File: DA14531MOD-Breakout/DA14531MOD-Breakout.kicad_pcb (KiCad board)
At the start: 2 copper layers, 30.1 x 30 mm, 3 parts, among them J1 Conn_01x07, J2 Conn_01x07, U1 DA14531MOD-00F01002

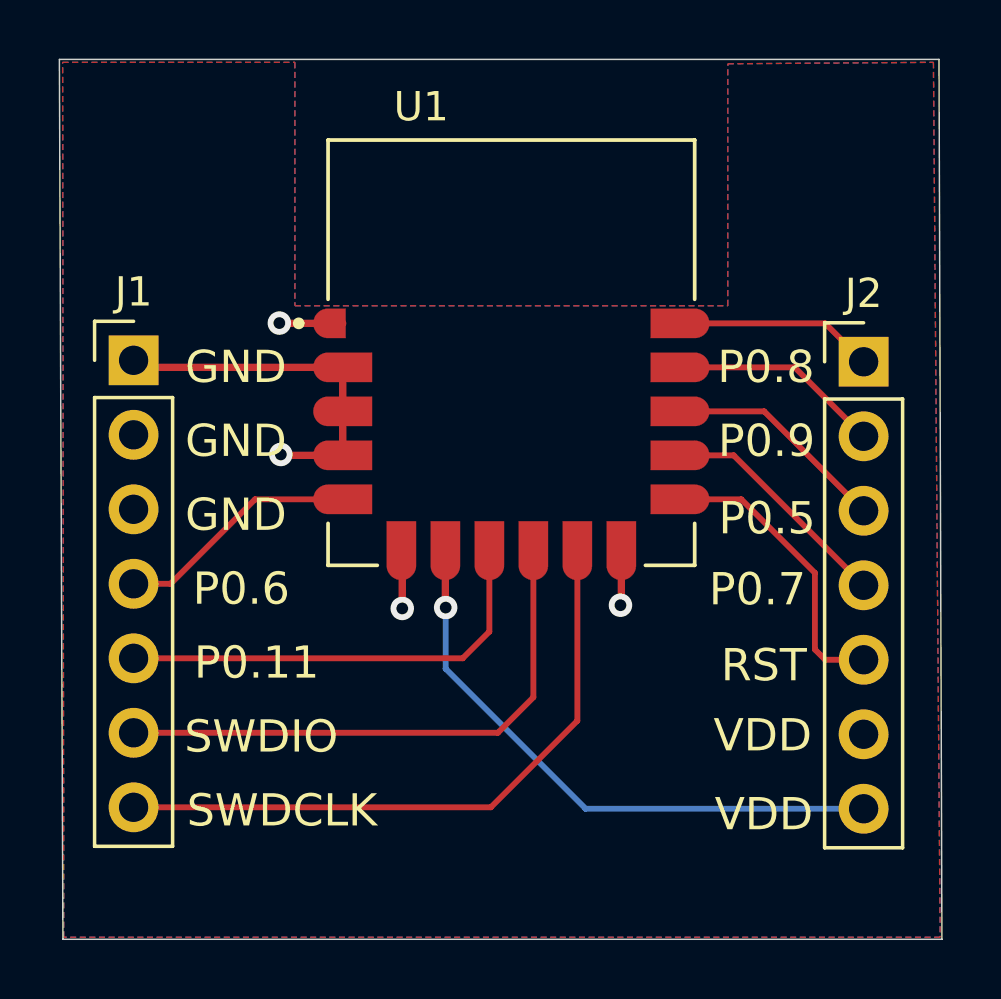
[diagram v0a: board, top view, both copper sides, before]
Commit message: finetuning
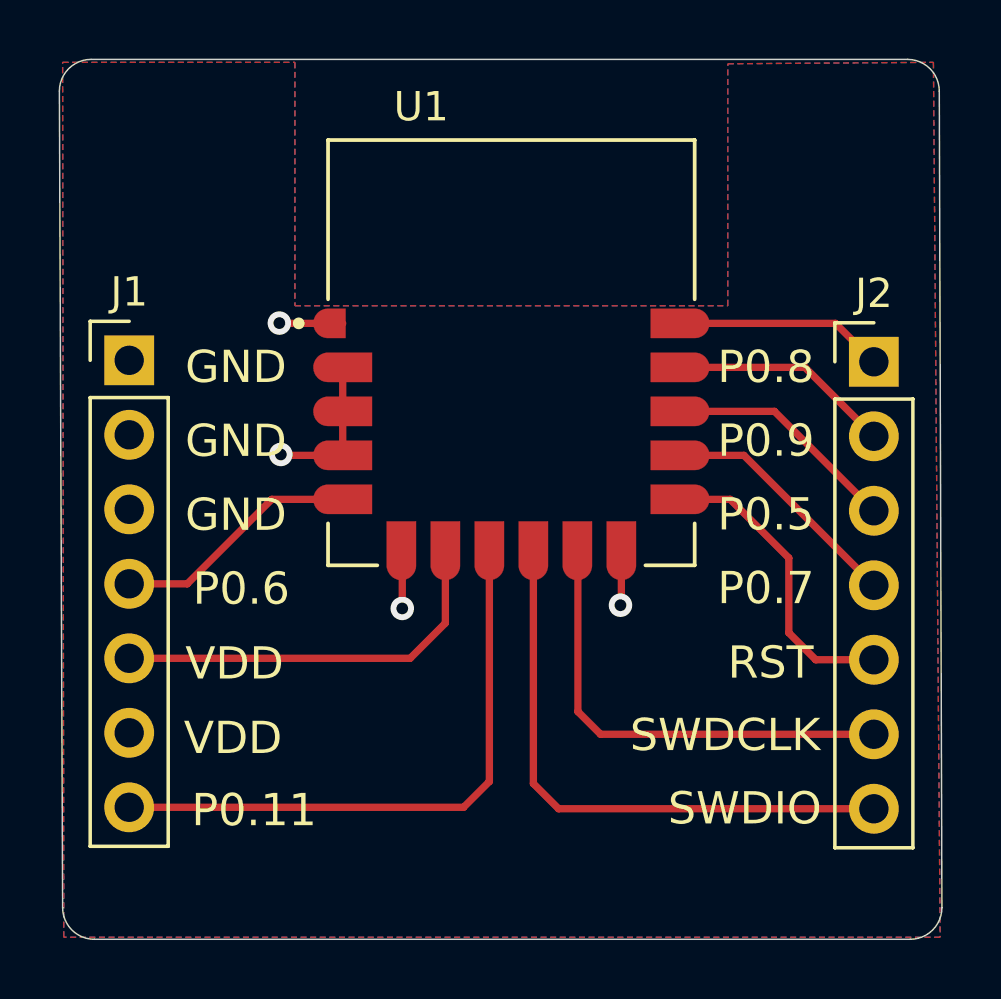
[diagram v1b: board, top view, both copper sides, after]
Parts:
- moved J2 0.35 mm to (103.7, 80.4)
- moved J1 0.15 mm to (78.3, 80.3)
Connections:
- J1 pad 5: /J8_P0_11 -> VDD
- J1 pad 6: /J9_P010_SWDIO -> VDD
- J1 pad 7: /J10_P02_SWDCLK -> /J8_P0_11
- J2 pad 6: VDD -> /J10_P02_SWDCLK
- J2 pad 7: VDD -> /J9_P010_SWDIO
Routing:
- net GND: track 18.4 -> 11.5 mm
- net VDD: track 20.3 -> 13.7 mm, vias 1 -> 0
- net /J10_P02_SWDCLK: track 22.2 -> 15.9 mm
- net /J8_P0_11: track 15.3 -> 20.5 mm
- net /J9_P010_SWDIO: track 19.1 -> 19.9 mm
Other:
- outline, holes or cut-outs redrawn

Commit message: kicad v7
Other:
- net class Default removed
